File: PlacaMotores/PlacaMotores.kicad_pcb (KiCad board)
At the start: 2 copper layers, 104.5 x 81.9 mm, 56 parts, among them J1 Screw_Terminal_01x04, J2 Conn_01x03_Male, J3 Conn_01x03_Male, J4 Conn_01x04_Male, J5 Conn_01x04_Male, U1 STA6940M, U5 LM311, U6 LM311

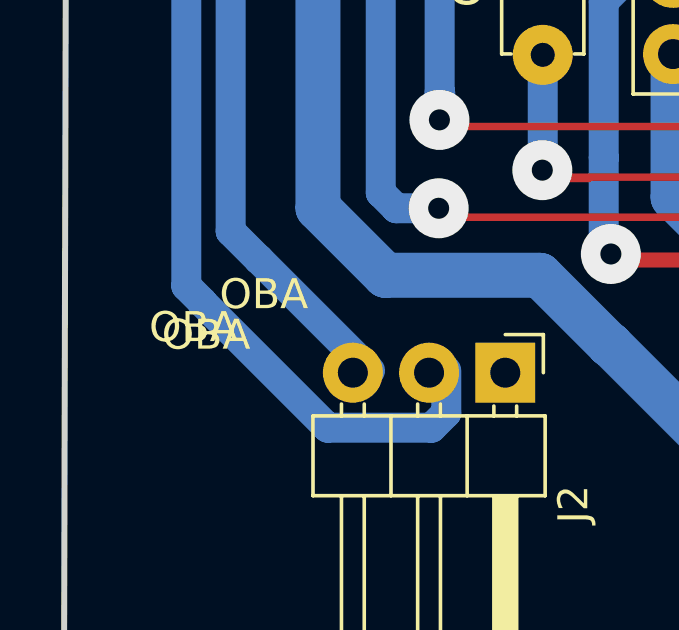
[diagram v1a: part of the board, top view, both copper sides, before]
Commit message: Imagen Esquematico agregada
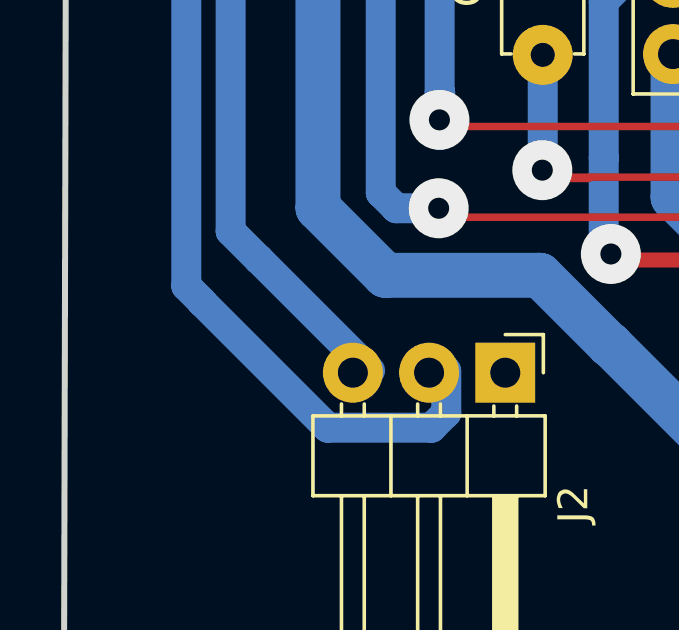
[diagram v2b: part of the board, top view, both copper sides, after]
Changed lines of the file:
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@@
   (general
     (thickness 1.6)
-    (drawings 43)
+    (drawings 36)
     (tracks 705)
     (zones 0)
@@
   (layers
     (0 F.Cu signal)
-    (31 B.Cu signal)
+    (31 B.Cu signal hide)
     (32 B.Adhes user hide)
     (33 F.Adhes user hide)
     (34 B.Paste user hide)
     (35 F.Paste user hide)
-    (36 B.SilkS user hide)
-    (37 F.SilkS user hide)
+    (36 B.SilkS user)
+    (37 F.SilkS user)
     (38 B.Mask user hide)
     (39 F.Mask user hide)
@@
     (45 Margin user hide)
     (46 B.CrtYd user hide)
-    (47 F.CrtYd user hide)
+    (47 F.CrtYd user)
     (48 B.Fab user hide)
     (49 F.Fab user)
@@
     )
   )
+  (dimension 104.201148 (width 0.3) (layer F.SilkS)
+    (gr_text "104,201 mm" (at 166.650486 70.002608 0.108937827) (layer F.SilkS)
+      (effects (font (size 1.5 1.5) (thickness 0.3)))
+    )
+    (feature1 (pts (xy 218.75496 72.00392) (xy 218.753844 71.417124)))
+    (feature2 (pts (xy 114.554 72.20204) (xy 114.552884 71.615244)))
+    (crossbar (pts (xy 114.553999 72.201664) (xy 218.754959 72.003544)))
+    (arrow1a (pts (xy 218.754959 72.003544) (xy 217.629572 72.592106)))
+    (arrow1b (pts (xy 218.754959 72.003544) (xy 217.627342 71.419266)))
+    (arrow2a (pts (xy 114.553999 72.201664) (xy 115.681616 72.785942)))
+    (arrow2b (pts (xy 114.553999 72.201664) (xy 115.679386 71.613102)))
+  )
+  (dimension 82.13852 (width 0.3) (layer F.SilkS)
+    (gr_text "82,139 mm" (at 107.53148 117.86362 270) (layer F.SilkS)
+      (effects (font (size 1.5 1.5) (thickness 0.3)))
+    )
+    (feature1 (pts (xy 109.63148 158.93288) (xy 109.045059 158.93288)))
+    (feature2 (pts (xy 109.63148 76.79436) (xy 109.045059 76.79436)))
+    (crossbar (pts (xy 109.63148 76.79436) (xy 109.63148 158.93288)))
+    (arrow1a (pts (xy 109.63148 158.93288) (xy 109.045059 157.806376)))
+    (arrow1b (pts (xy 109.63148 158.93288) (xy 110.217901 157.806376)))
+    (arrow2a (pts (xy 109.63148 76.79436) (xy 109.045059 77.920864)))
+    (arrow2b (pts (xy 109.63148 76.79436) (xy 110.217901 77.920864)))
+  )
   (gr_text VBB (at 174.833948 92.299923 90) (layer F.Fab)
     (effects (font (size 1 1) (thickness 0.25)))
@@
     (effects (font (size 1 1) (thickness 0.25)))
   )
-  (gr_text OBA (at 120.8278 145.93824) (layer F.SilkS)
-    (effects (font (size 1 1) (thickness 0.25)))
-  )
-  (gr_text OBA (at 118.48084 147.03552) (layer F.SilkS)
-    (effects (font (size 1 1) (thickness 0.25)))
-  )
-  (gr_text OBA (at 118.90248 147.28952) (layer F.SilkS)
-    (effects (font (size 1 1) (thickness 0.25)))
-  )
   (gr_text OBB (at 189.929168 146.915003 90) (layer F.Fab)
     (effects (font (size 1 1) (thickness 0.25)))
@@
   (gr_line (start 218.622482 76.649822) (end 114.325002 76.863182) (layer Edge.Cuts) (width 0.2))
   (gr_line (start 218.541202 157.574222) (end 218.668202 77.218782) (layer Edge.Cuts) (width 0.2))
-  (dimension 105.54697 (width 0.3) (layer B.SilkS)
-    (gr_text "105,547 mm" (at 167.250419 69.260236 0.55154033) (layer B.SilkS)
-      (effects (font (size 1.5 1.5) (thickness 0.3)))
-    )
-    (feature1 (pts (xy 114.499594 71.868139) (xy 114.493949 71.281745)))
-    (feature2 (pts (xy 220.041674 70.852139) (xy 220.036029 70.265745)))
-    (crossbar (pts (xy 220.041674 70.852139) (xy 114.499594 71.868139)))
-    (arrow1a (pts (xy 114.499594 71.868139) (xy 115.620401 71.270902)))
-    (arrow1b (pts (xy 114.499594 71.868139) (xy 115.63169 72.443689)))
-    (arrow2a (pts (xy 220.041674 70.852139) (xy 218.909578 70.276589)))
-    (arrow2b (pts (xy 220.041674 70.852139) (xy 218.920867 71.449376)))
-  )
-  (dimension 5.183156 (width 0.3) (layer B.SilkS)
-    (gr_text "5,183 mm" (at 194.549024 100.738434 88.5959728) (layer B.SilkS)
-      (effects (font (size 1.5 1.5) (thickness 0.3)))
-    )
-    (feature1 (pts (xy 192.513154 98.096179) (xy 193.099399 98.110548)))
-    (feature2 (pts (xy 192.386154 103.277779) (xy 192.972399 103.292148)))
-    (crossbar (pts (xy 192.386154 103.277779) (xy 192.513154 98.096179)))
-    (arrow1a (pts (xy 192.513154 98.096179) (xy 193.071797 99.236713)))
-    (arrow1b (pts (xy 192.513154 98.096179) (xy 191.899307 99.207976)))
-    (arrow2a (pts (xy 192.386154 103.277779) (xy 193.000001 102.165982)))
-    (arrow2b (pts (xy 192.386154 103.277779) (xy 191.827511 102.137245)))
-  )
-  (dimension 7.137445 (width 0.3) (layer B.SilkS)
-    (gr_text "7,137 mm" (at 185.86796 106.231234 0.20389871) (layer B.SilkS)
-      (effects (font (size 1.5 1.5) (thickness 0.3)))
-    )
-    (feature1 (pts (xy 182.276954 99.975779) (xy 182.293874 104.730364)))
-    (feature2 (pts (xy 189.414354 99.950379) (xy 189.431274 104.704964)))
-    (crossbar (pts (xy 189.429187 104.118547) (xy 182.291787 104.143947)))
-    (arrow1a (pts (xy 182.291787 104.143947) (xy 183.416197 103.553521)))
-    (arrow1b (pts (xy 182.291787 104.143947) (xy 183.420371 104.726355)))
-    (arrow2a (pts (xy 189.429187 104.118547) (xy 188.300603 103.536139)))
-    (arrow2b (pts (xy 189.429187 104.118547) (xy 188.304777 104.708973)))
-  )
-  (dimension 5.032342 (width 0.3) (layer B.SilkS)
-    (gr_text "5,032 mm" (at 213.850672 105.872694 -87.97523492) (layer B.SilkS)
-      (effects (font (size 1.5 1.5) (thickness 0.3)))
-    )
-    (feature1 (pts (xy 216.211354 108.306979) (xy 215.452207 108.333818)))
-    (feature2 (pts (xy 216.033554 103.277779) (xy 215.274407 103.304618)))
-    (crossbar (pts (xy 215.860461 103.283898) (xy 216.038261 108.313098)))
-    (arrow1a (pts (xy 216.038261 108.313098) (xy 215.412405 107.208017)))
-    (arrow1b (pts (xy 216.038261 108.313098) (xy 216.584515 107.166578)))
-    (arrow2a (pts (xy 215.860461 103.283898) (xy 215.314207 104.430418)))
-    (arrow2b (pts (xy 215.860461 103.283898) (xy 216.486317 104.388979)))
-  )
-  (dimension 13.690812 (width 0.3) (layer B.SilkS)
-    (gr_text "13,691 mm" (at 206.634542 103.155246 0.3188971) (layer B.SilkS)
-      (effects (font (size 1.5 1.5) (thickness 0.3)))
-    )
-    (feature1 (pts (xy 213.468154 101.017179) (xy 213.471418 101.603591)))
-    (feature2 (pts (xy 199.777554 101.093379) (xy 199.780818 101.679791)))
-    (crossbar (pts (xy 199.777554 101.093379) (xy 213.468154 101.017179)))
-    (arrow1a (pts (xy 213.468154 101.017179) (xy 212.344932 101.609861)))
-    (arrow1b (pts (xy 213.468154 101.017179) (xy 212.338404 100.437037)))
-    (arrow2a (pts (xy 199.777554 101.093379) (xy 200.907304 101.673521)))
-    (arrow2b (pts (xy 199.777554 101.093379) (xy 200.900776 100.500697)))
-  )
   (dimension 79.934882 (width 0.3) (layer Cmts.User)
     (gr_text "79,935 mm" (at 175.358315 166.720489 1.474867464) (layer Cmts.User)
@@
     (arrow2b (pts (xy 135.458166 169.848493) (xy 136.569203 169.233272)))
   )
-  (dimension 5.080063 (width 0.3) (layer B.SilkS)
-    (gr_text "5,080 mm" (at 125.863219 101.016849 89.7135235) (layer B.SilkS)
-      (effects (font (size 1.5 1.5) (thickness 0.3)))
-    )
-    (feature1 (pts (xy 128.20563 98.488498) (xy 127.389479 98.484417)))
-    (feature2 (pts (xy 128.18023 103.568498) (xy 127.364079 103.564417)))
-    (crossbar (pts (xy 127.950493 103.567349) (xy 127.975893 98.487349)))
-    (arrow1a (pts (xy 127.975893 98.487349) (xy 128.556674 99.616771)))
-    (arrow1b (pts (xy 127.975893 98.487349) (xy 127.383847 99.610907)))
-    (arrow2a (pts (xy 127.950493 103.567349) (xy 128.542539 102.443791)))
-    (arrow2b (pts (xy 127.950493 103.567349) (xy 127.369712 102.437927)))
-  )
   (via (at 130.108562 141.800822) (size 2) (drill 0.7) (layers F.Cu B.Cu) (net 1))
